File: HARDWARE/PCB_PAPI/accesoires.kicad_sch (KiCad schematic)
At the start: 21 parts, among them IC5 ADXL343BCCZ-RL, IC6 MAX98357AETE+, IC7 W25Q128JVPIQ_TR

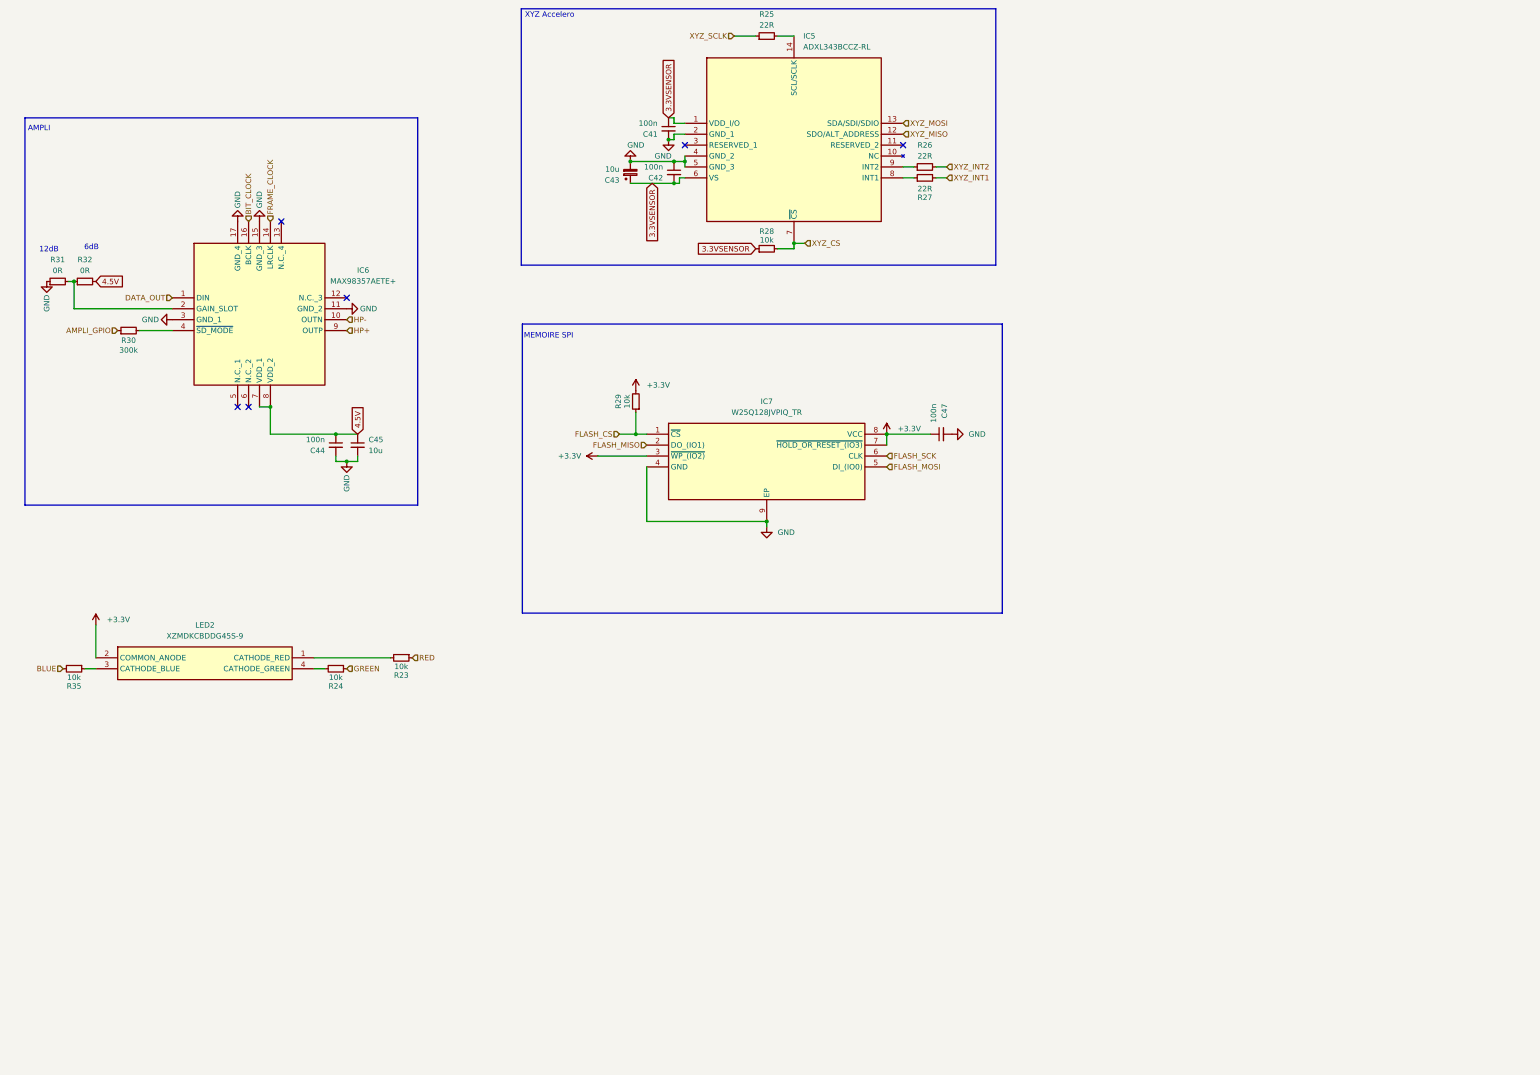
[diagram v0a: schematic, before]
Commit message: update
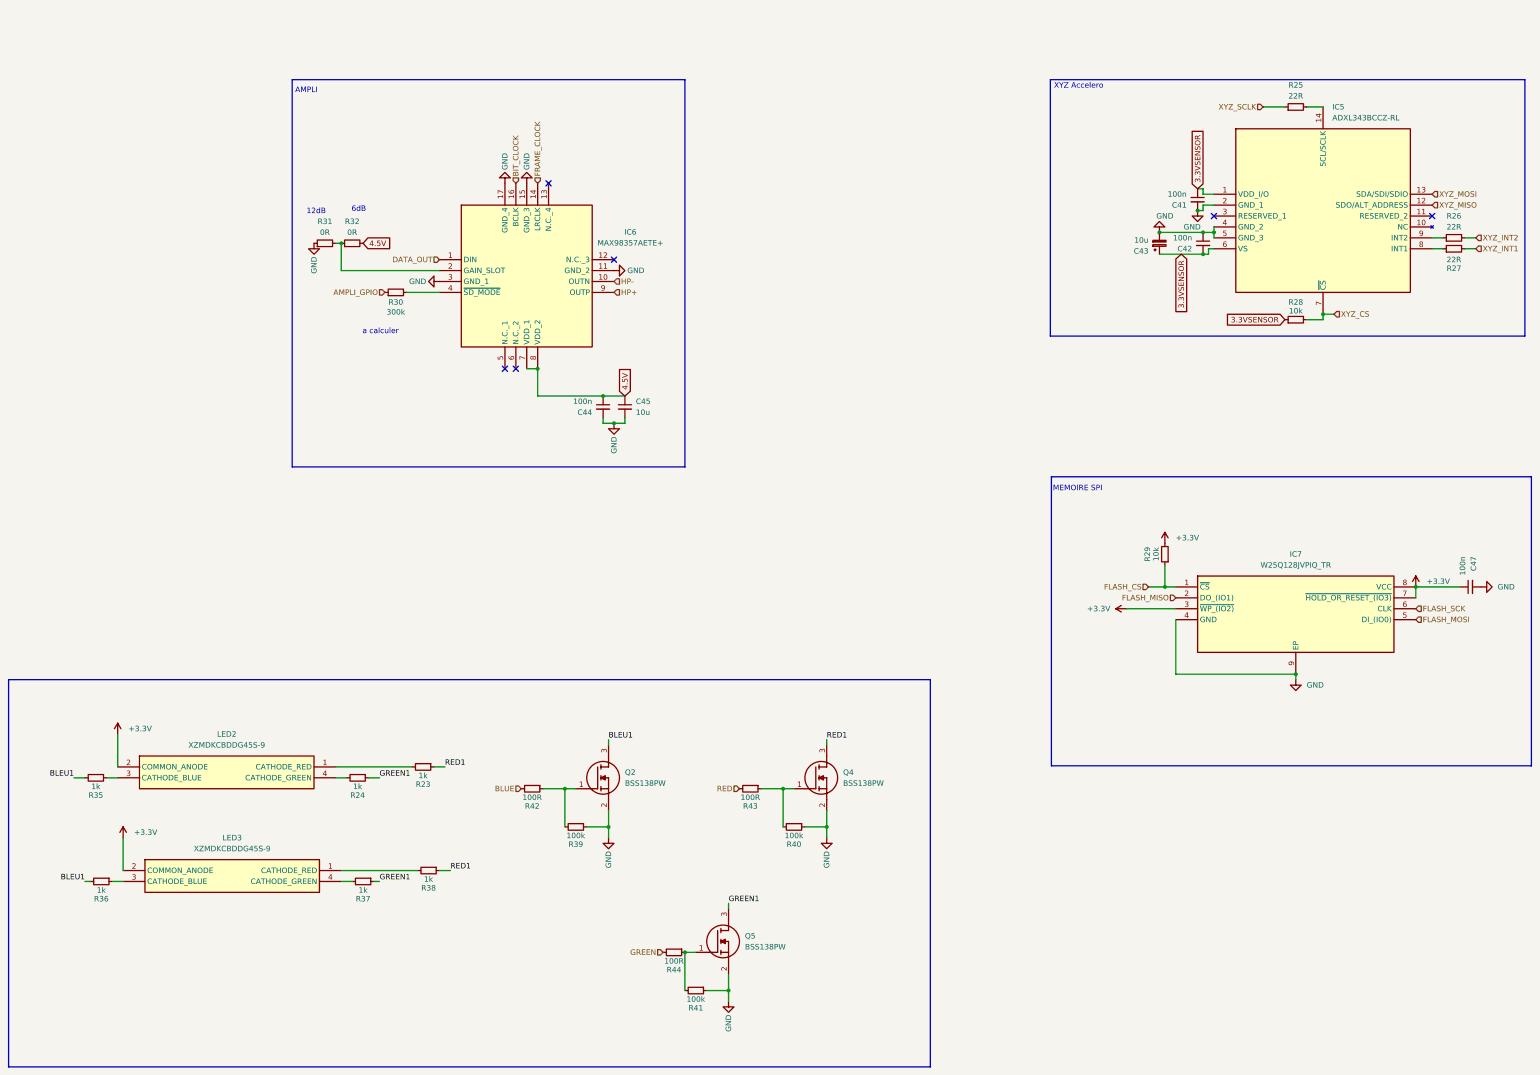
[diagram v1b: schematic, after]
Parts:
- added LED3: XZMDKCBDDG45S-9, samacsys:XZMDKCBDDG45S9, symbol samacsys:XZMDKCBDDG45S-9
- added Q2, Q4, Q5: BSS138PW, samacsys:SOT65P210X110-3N, symbol samacsys:BSS138PW
- added R36, R37, R38: 1k, Resistor_SMD:R_0201_0603Metric, symbol Device:R_Small
- added R39, R40, R41: 100k, Resistor_SMD:R_0201_0603Metric, symbol Device:R_Small
- added R42, R43, R44: 100R, Resistor_SMD:R_0201_0603Metric, symbol Device:R_Small
- LED2: footprint XZMDKCBDDG45S9 -> samacsys:XZMDKCBDDG45S9
- R23, R24, R35: value 10k -> 1k
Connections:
- net +3.3V: now also LED3.2 (COMMON_ANODE)
- net BLUE: now also R42.2; no longer R35.2
- net GND: now also Q2.2 (S), Q4.2 (S), Q5.2 (S), R39.1, R40.1, R41.1
- net GREEN: now also R44.2; no longer R24.1
- net RED: now also R43.2; no longer R23.1
- new net: Q5.1 (G), R41.2, R44.1
- new net: Q2.1 (G), R39.2, R42.1
- new net: LED3.3 (CATHODE_BLUE), R36.1
- new net: LED3.1 (CATHODE_RED), R38.2
- new net: LED3.4 (CATHODE_GREEN), R37.2
- new net: Q4.1 (G), R40.2, R43.1
- new net BLEU1: Q2.3 (D), R35.2, R36.2
- new net GREEN1: Q5.3 (D), R24.1, R37.1
- new net RED1: Q4.3 (D), R23.1, R38.1
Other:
- note added: "a calculer"
- moved on the sheet: C41, C42, C43, C44, C45, C47, IC5, IC6, IC7, LED2, R23, R24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
